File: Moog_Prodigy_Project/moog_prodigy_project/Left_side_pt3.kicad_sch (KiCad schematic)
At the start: 55 parts, among them SW7 SW_Slide_DPDT, SW9 SW_DPDT_x2, U12B MCP6562, U13B MCP6562, U14 AD8001AR, U14C BF244A, U14E 4007, U15 AD8001AR, U4 AD8001AR

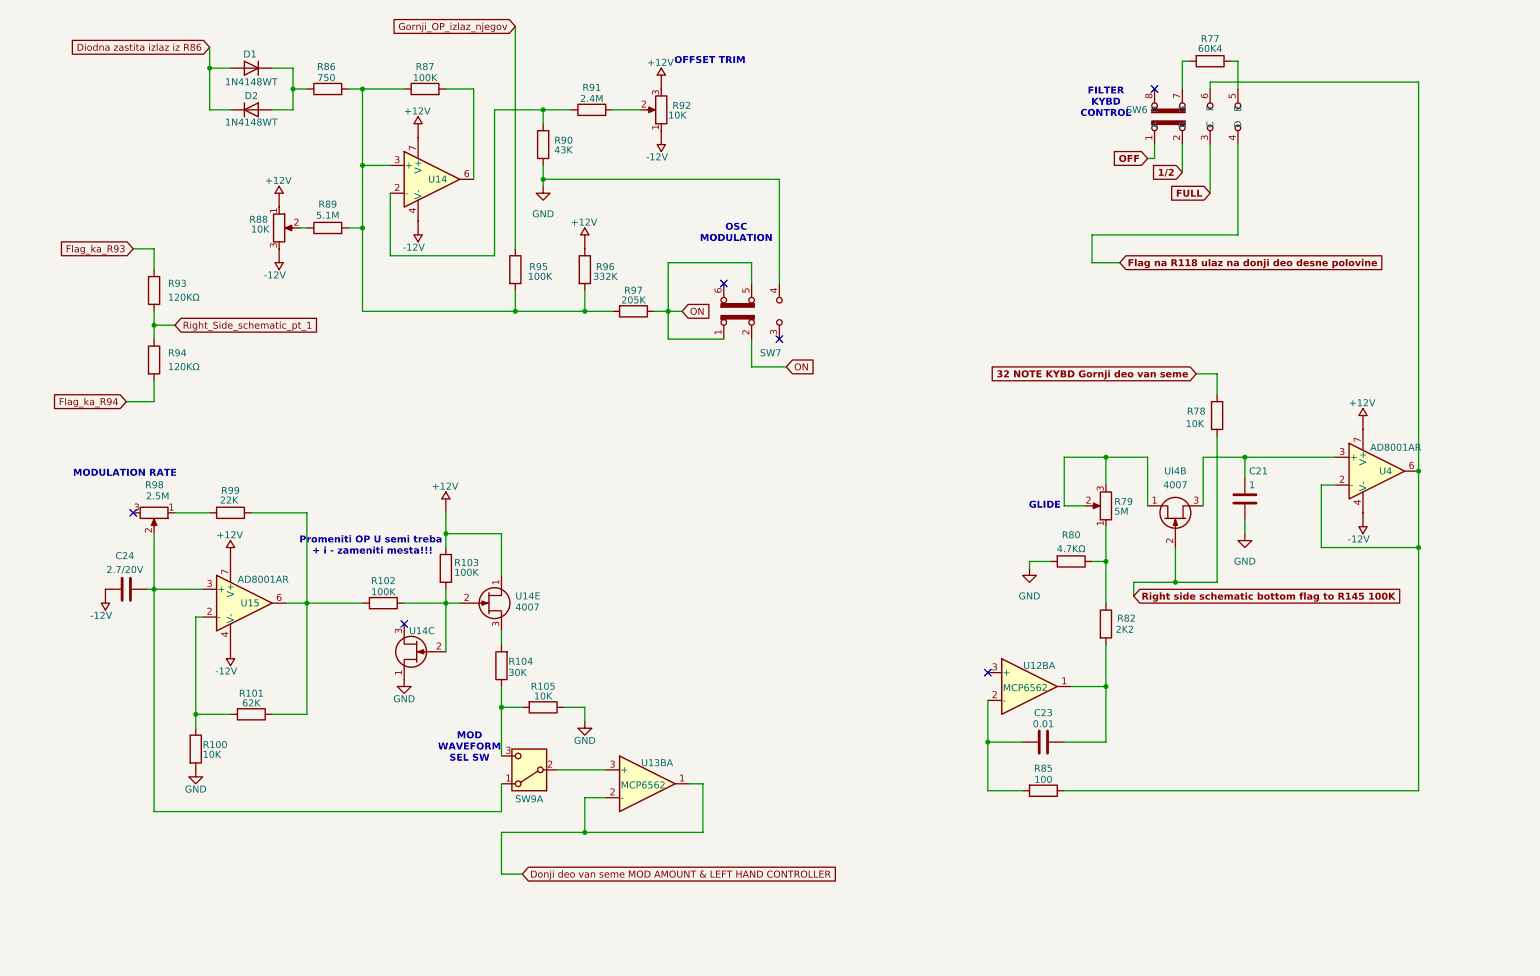
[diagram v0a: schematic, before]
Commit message: Imoprt LF393 & Sortiranje fleg-ova 07.04.2026
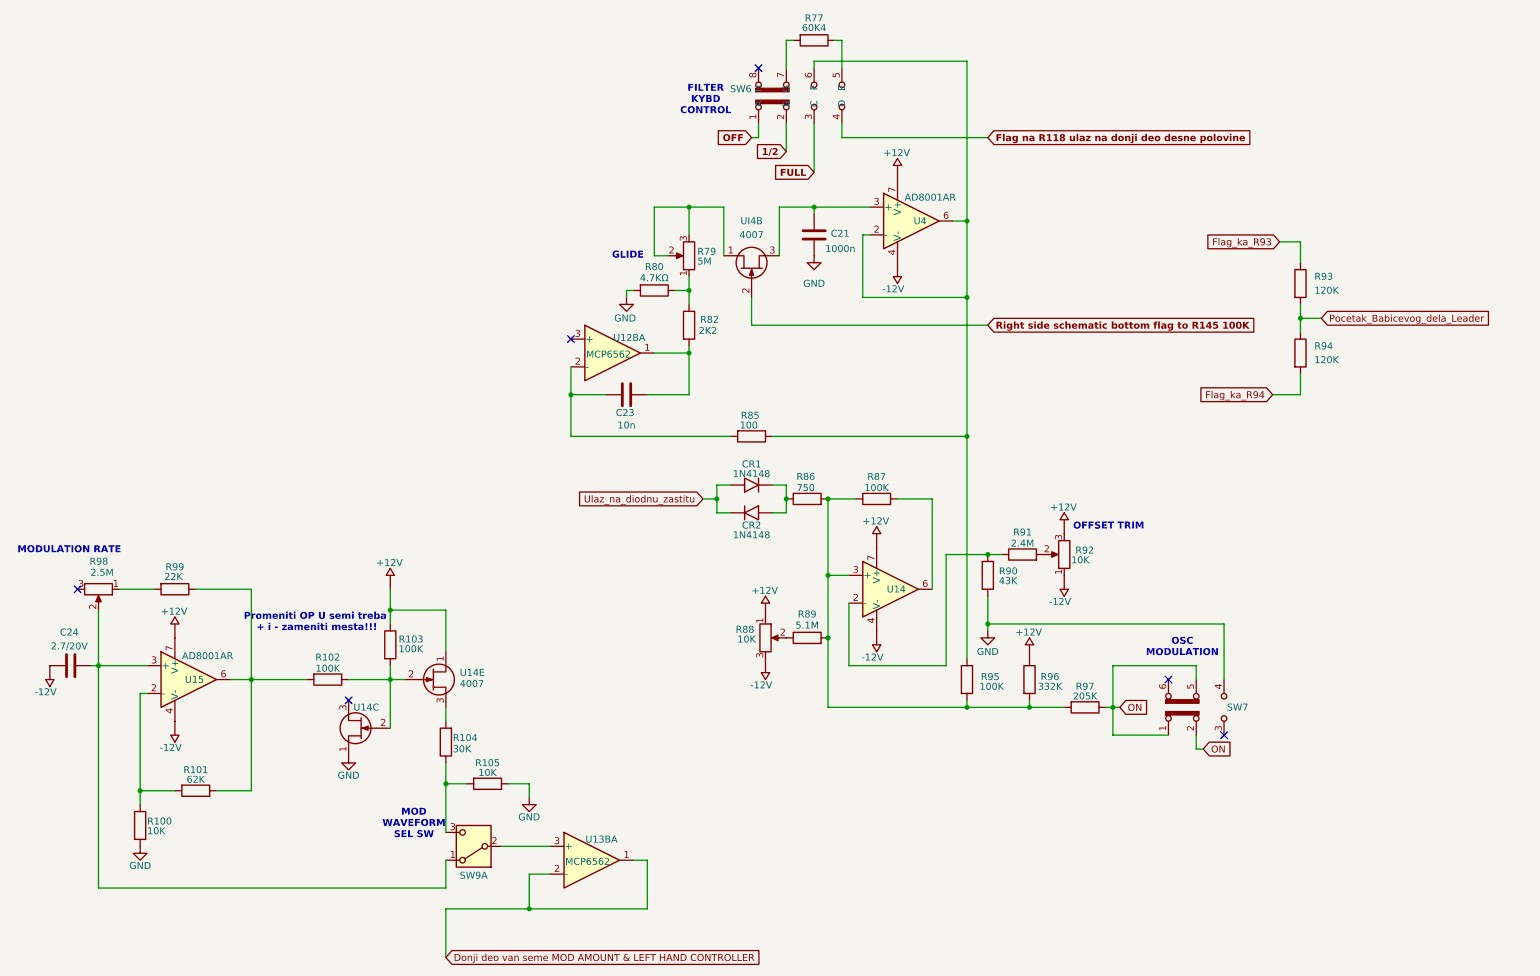
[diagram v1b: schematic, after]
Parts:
- removed D1, D2: 1N4148WT, Diode_SMD:D_SOD-523, symbol Diode:1N4148WT
- removed R78: 10K, symbol Device:R
- added CR1, CR2: 1N4148, Diode_THT:D_DO-35_SOD27_P7.62mm_Horizontal, symbol Diode:1N4148
- C21: value 1 -> 1000n
- C23: value 0.01 -> 10n
- R93, R94: value 120KΩ -> 120K
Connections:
- net Gornji_OP_izlaz_njegov is gone; now on an unnamed net: R95.1
- net at R86.1: now also CR1.1 (K), CR2.2 (A)
- net Right_Side_schematic_pt_1 renamed Pocetak_Babicevog_dela_Leader
- new net Ulaz_na_diodnu_zastitu: CR1.2 (A), CR2.1 (K)
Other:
- moved on the sheet: C21, C23, C24, R100, R101, R102, R103, R104, R105, R77, R79, R80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
